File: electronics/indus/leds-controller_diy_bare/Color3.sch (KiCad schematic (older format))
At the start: 18 parts, among them U2 TPS92513HVDGQT

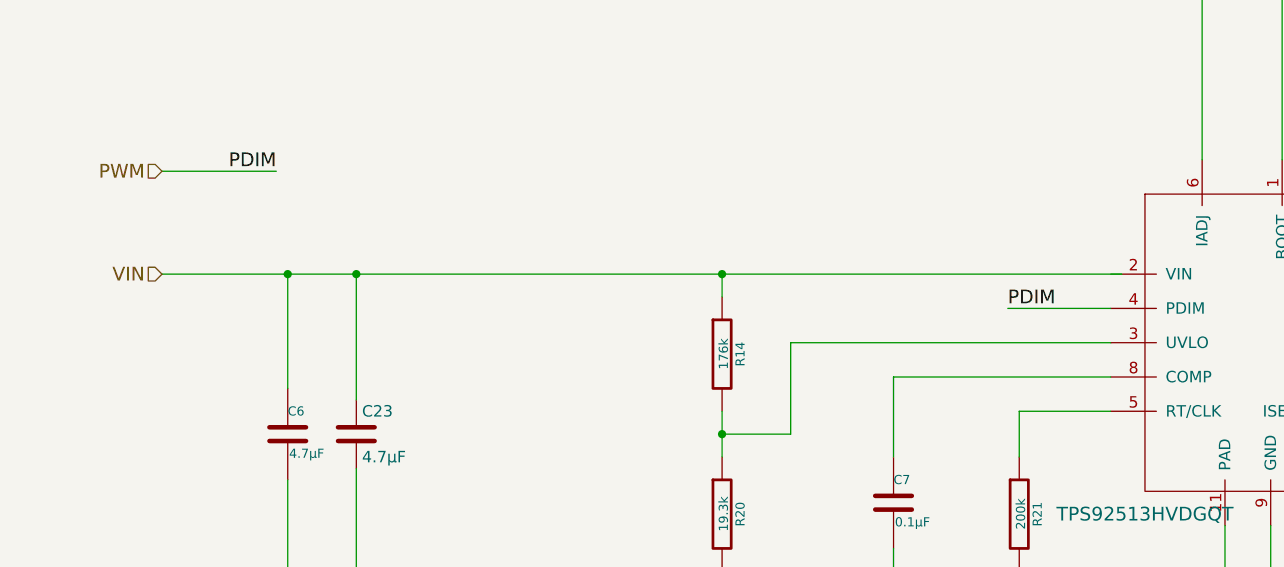
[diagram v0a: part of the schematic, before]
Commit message: fix some errors
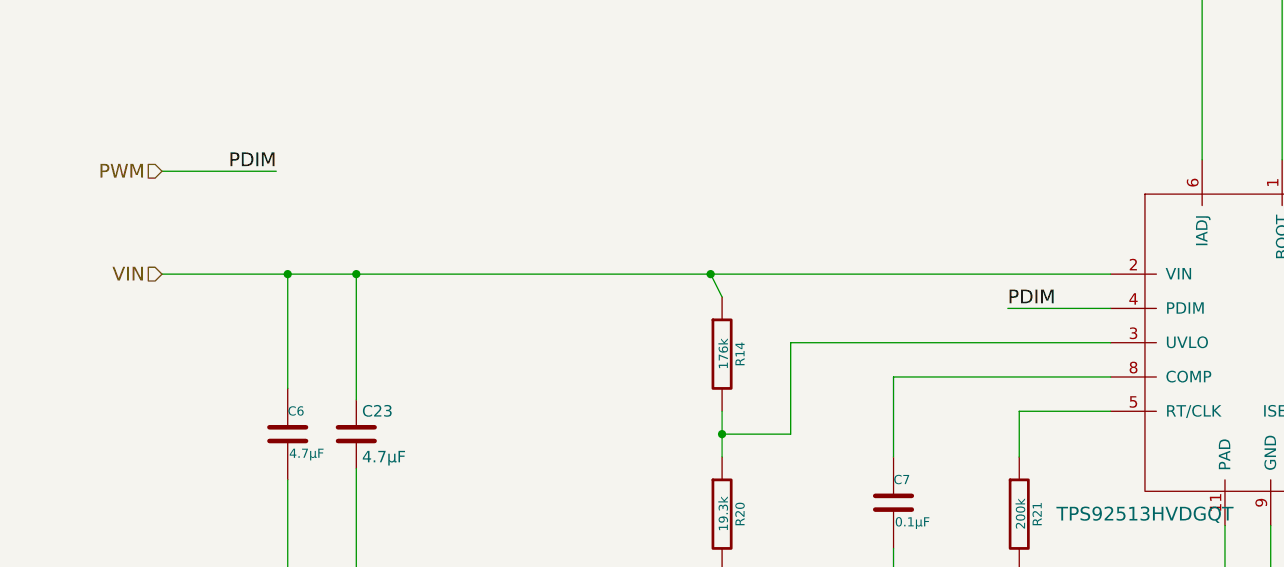
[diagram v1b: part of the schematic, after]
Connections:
- net VIN: now also U2.2 (VIN)
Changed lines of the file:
@@
 POT_OUT
 Wire Wire Line
-	1200 3850 5400 3850
+	1200 3850 5350 3850
 Wire Wire Line
 	1750 5300 10250 5300
@@
 	3650 5150 3650 5300
 Wire Wire Line
-	3650 3950 3650 3850
-Connection ~ 3650 3850
+	3650 3950 3600 3850
+Connection ~ 3600 3850
 Connection ~ 3650 5300
 Wire Wire Line
